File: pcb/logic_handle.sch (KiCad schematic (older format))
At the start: 18 parts, among them U1 NCP1117-3.3_TO252

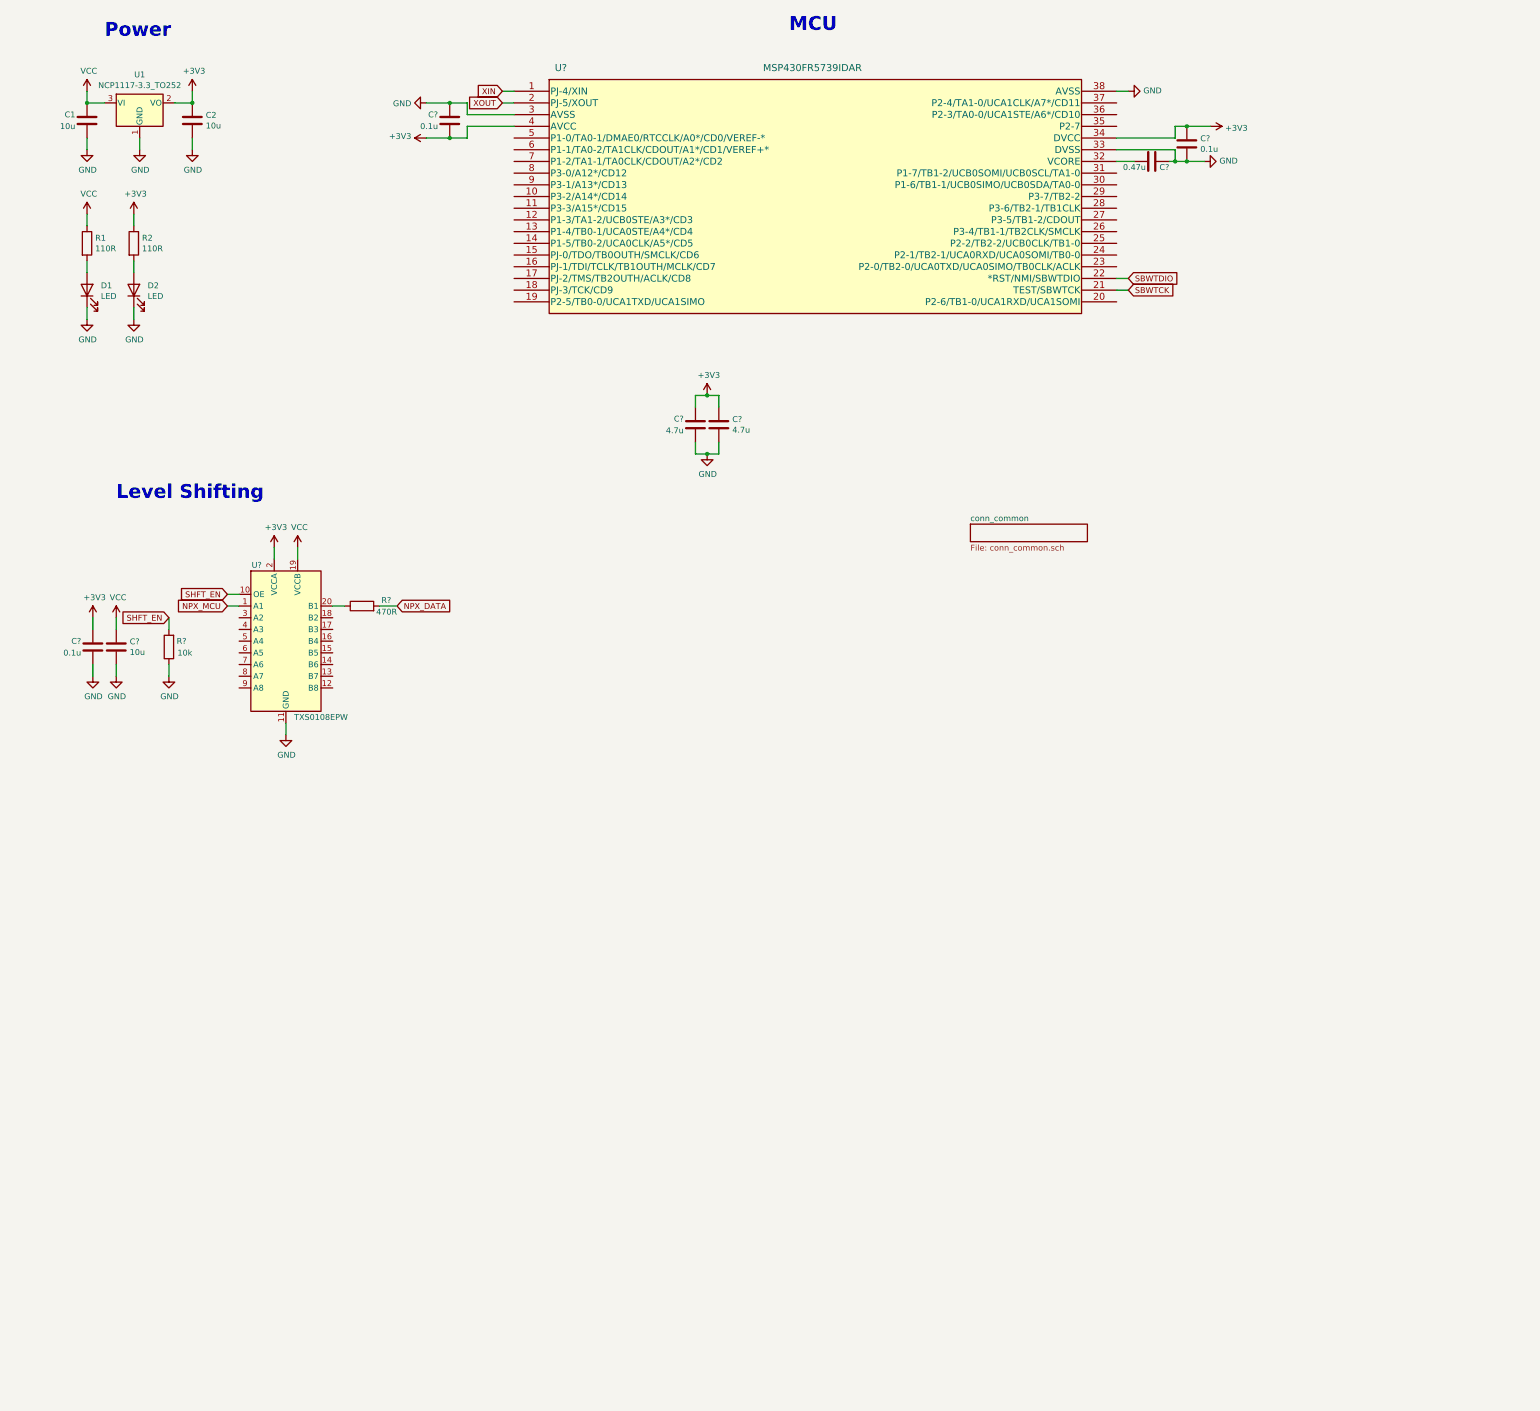
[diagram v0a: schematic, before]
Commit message: [WIP]: Logic handle schematic and layout complete
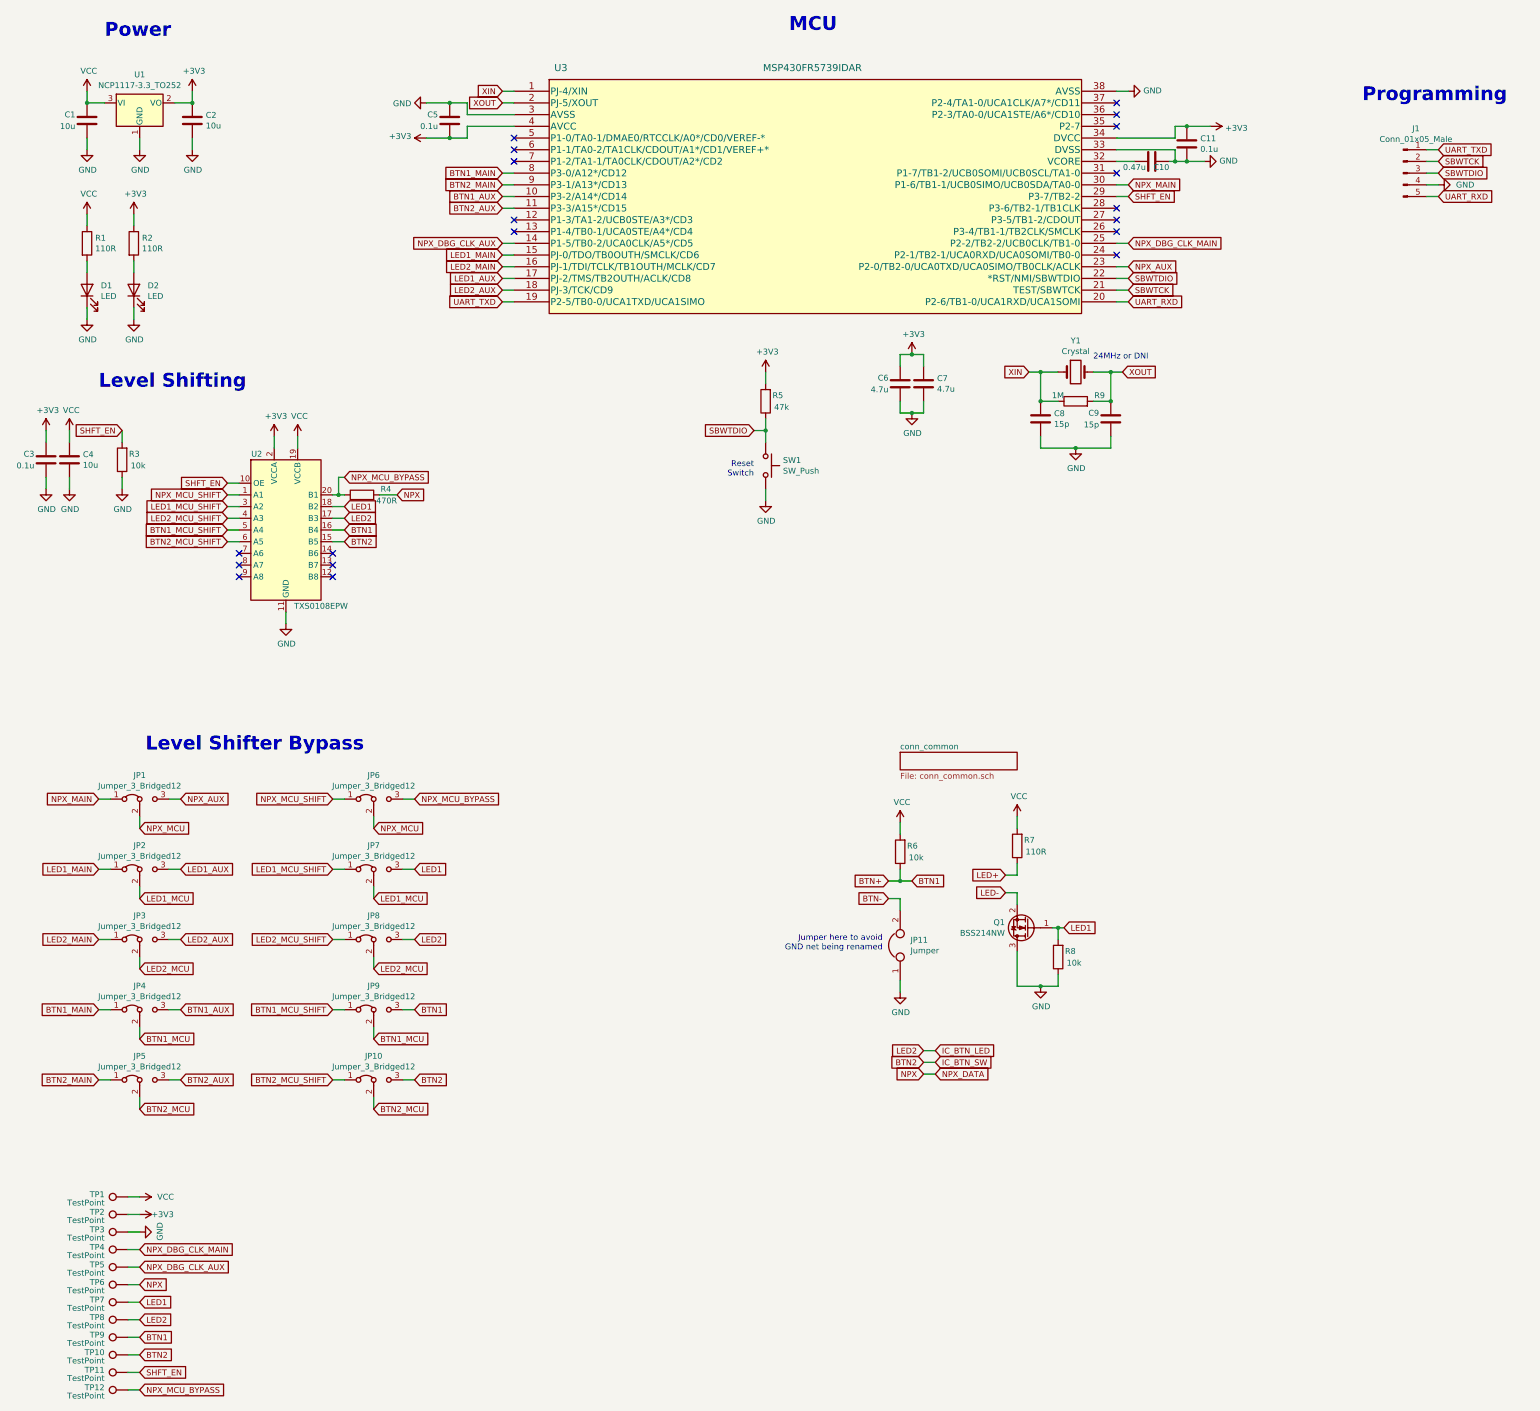
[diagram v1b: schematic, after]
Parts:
- added C8, C9: 15p, Capacitor_SMD:C_0805_2012Metric, symbol Device:C
- added J1: Conn_01x05_Male, Connector_PinHeader_2.54mm:PinHeader_1x05_P2.54mm_Vertical, symbol Connector:Conn_01x05_Male
- added JP1, JP10, JP2, JP3, JP4, JP5, JP6, JP7, JP8, JP9: Jumper_3_Bridged12, Jumper:SolderJumper-3_P1.3mm_Bridged2Bar12_Pad1.0x1.5mm, symbol Jumper:Jumper_3_Bridged12
- added JP11: Jumper, Jumper:SolderJumper-2_P1.3mm_Bridged2Bar_Pad1.0x1.5mm, symbol Device:Jumper
- added Q1: BSS214NW, Package_TO_SOT_SMD:SOT-323_SC-70, symbol Transistor_FET:BSS214NW
- added R5: 47k, Resistor_SMD:R_0805_2012Metric, symbol Device:R
- added R6, R8: 10k, Resistor_SMD:R_0805_2012Metric, symbol Device:R
- added R7: 110R, Resistor_SMD:R_0805_2012Metric, symbol Device:R
- added R9: 1M, Resistor_SMD:R_0805_2012Metric, symbol Device:R
- added SW1: SW_Push, Button_Switch_SMD:SW_SPST_TL3342, symbol Switch:SW_Push
- added TP1, TP10, TP11, TP12, TP2, TP3, TP4, TP5, TP6, TP7, TP8, TP9: TestPoint, TestPoint:TestPoint_Pad_2.0x2.0mm, symbol Connector:TestPoint
- added Y1: Crystal, Gigahawk:Crystal_SMD_AWSZT-CV-2Pin_3.7x3.1mm, symbol Device:Crystal
- C1, C2: footprint (none) -> Capacitor_SMD:C_0805_2012Metric
- C10, C11, C3, C4, C5, C6, C7: renamed from C?; footprint (none) -> Capacitor_SMD:C_0805_2012Metric
- R1, R2: footprint (none) -> Resistor_SMD:R_0805_2012Metric
- R3, R4: renamed from R?; footprint (none) -> Resistor_SMD:R_0805_2012Metric
- gave numbers to parts that had none: 2
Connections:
- net +3V3: now also R5.2, TP2.1
- net GND: now also C8.2, C9.1, J1.4 (Pin_4), JP11.1, Q1.3 (D), R8.1, SW1.2, TP3.1
- net NPX_MCU: now also JP1.2 (C), JP6.2 (C); no longer U2.1 (A1)
- net SBWTCK: now also J1.2 (Pin_2)
- net SBWTDIO: now also J1.3 (Pin_3), R5.1, SW1.1
- net SHFT_EN: now also U3.29 (P3-7/TB2-2), TP11.1
- net VCC: now also R6.2, R7.2, TP1.1
- net XIN: now also C8.1, R9.1, Y1.1
- net XOUT: now also C9.2, R9.2, Y1.2
- net BTN1_AUX: now reaches U3.10 (P3-2/A14*/CD14)
- net BTN1_AUX: now also JP4.3 (B)
- net BTN2_AUX: now reaches U3.11 (P3-3/A15*/CD15)
- net BTN2_AUX: now also JP5.3 (B)
- net NPX_DBG_CLK_AUX: now reaches U3.14 (P1-5/TB0-2/UCA0CLK/A5*/CD5)
- net NPX_DBG_CLK_AUX: now also TP5.1
- net LED1_MAIN: now reaches U3.15 (PJ-0/TDO/TB0OUTH/SMCLK/CD6)
- net LED1_MAIN: now also JP2.1 (A)
- net LED2_MAIN: now reaches U3.16 (PJ-1/TDI/TCLK/TB1OUTH/MCLK/CD7)
- net LED2_MAIN: now also JP3.1 (A)
- net LED1_AUX: now reaches U3.17 (PJ-2/TMS/TB2OUTH/ACLK/CD8)
- net LED1_AUX: now also JP2.3 (B)
- net LED2_AUX: now reaches U3.18 (PJ-3/TCK/CD9)
- net LED2_AUX: now also JP3.3 (B)
- net UART_TXD: now reaches U3.19 (P2-5/TB0-0/UCA1TXD/UCA1SIMO)
- net UART_TXD: now also J1.1 (Pin_1)
- net UART_RXD: now reaches U3.20 (P2-6/TB1-0/UCA1RXD/UCA1SOMI)
- net UART_RXD: now also J1.5 (Pin_5)
- net NPX_AUX: now reaches U3.23 (P2-0/TB2-0/UCA0TXD/UCA0SIMO/TB0CLK/ACLK)
- net NPX_AUX: now also JP1.3 (B)
- net NPX_DBG_CLK_MAIN: now reaches U3.25 (P2-2/TB2-2/UCB0CLK/TB1-0)
- net NPX_DBG_CLK_MAIN: now also TP4.1
- net NPX_MAIN: now reaches U3.30 (P1-6/TB1-1/UCB0SIMO/UCB0SDA/TA0-0)
- net NPX_MAIN: now also JP1.1 (A)
- net BTN1_MAIN: now reaches U3.8 (P3-0/A12*/CD12)
- net BTN1_MAIN: now also JP4.1 (A)
- net BTN2_MAIN: now reaches U3.9 (P3-1/A13*/CD13)
- net BTN2_MAIN: now also JP5.1 (A)
- net BTN2: now reaches U2.15 (B5)
- net BTN2: now also JP10.3 (B), TP10.1
- net BTN+: now reaches U2.16 (B4)
- net BTN+: now also JP9.3 (B), R6.1, TP9.1
- net IC_BTN_LED: now reaches U2.17 (B3)
- net IC_BTN_LED: now also JP8.3 (B), TP8.1
- net LED1: now reaches U2.18 (B2)
- net LED1: now also JP7.3 (B), Q1.1 (G), R8.2, TP7.1
- net NPX_MCU_BYPASS: now reaches R4.1, U2.20 (B1)
- net NPX_MCU_BYPASS: now also JP6.3 (B), TP12.1
- net LED1_MCU_SHIFT: now reaches U2.3 (A2)
- net LED1_MCU_SHIFT: now also JP7.1 (A)
- net LED2_MCU_SHIFT: now reaches U2.4 (A3)
- net LED2_MCU_SHIFT: now also JP8.1 (A)
- net BTN1_MCU_SHIFT: now reaches U2.5 (A4)
- net BTN1_MCU_SHIFT: now also JP9.1 (A)
- net BTN2_MCU_SHIFT: now reaches U2.6 (A5)
- net BTN2_MCU_SHIFT: now also JP10.1 (A)
- net NPX_DATA renamed NPX
- net NPX: now also TP6.1
- new net BTN-: JP11.2
- new net BTN1_MCU: JP4.2 (C), JP9.2 (C)
- new net BTN2_MCU: JP10.2 (C), JP5.2 (C)
- new net LED+: R7.1
- new net LED-: Q1.2 (S)
- new net LED1_MCU: JP2.2 (C), JP7.2 (C)
- new net LED2_MCU: JP3.2 (C), JP8.2 (C)
- new net NPX_MCU_SHIFT: JP6.1 (A), U2.1 (A1)
- no-connect marks 0 -> 19
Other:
- note added: "24MHz or DNI"
- note added: "Jumper here to avoid\nGND net being renamed"
- note added: "Level Shifter Bypass"
- note added: "Programming"
- note added: "Reset\nSwitch"
- moved on the sheet: C3, C4, C6, C7, R3, R4, U2
